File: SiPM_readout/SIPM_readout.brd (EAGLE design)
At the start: 57 x 37.5 mm, 28 parts

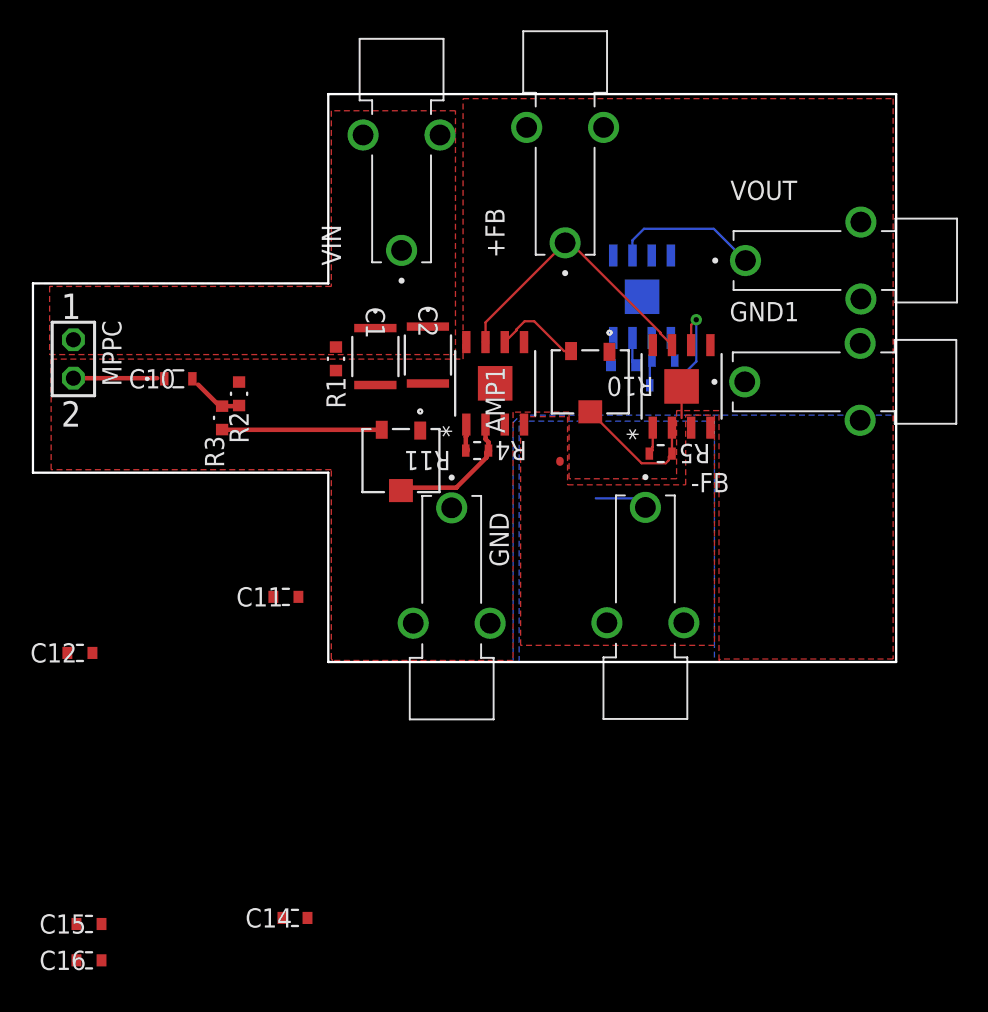
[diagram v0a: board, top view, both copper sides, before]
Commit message: compact
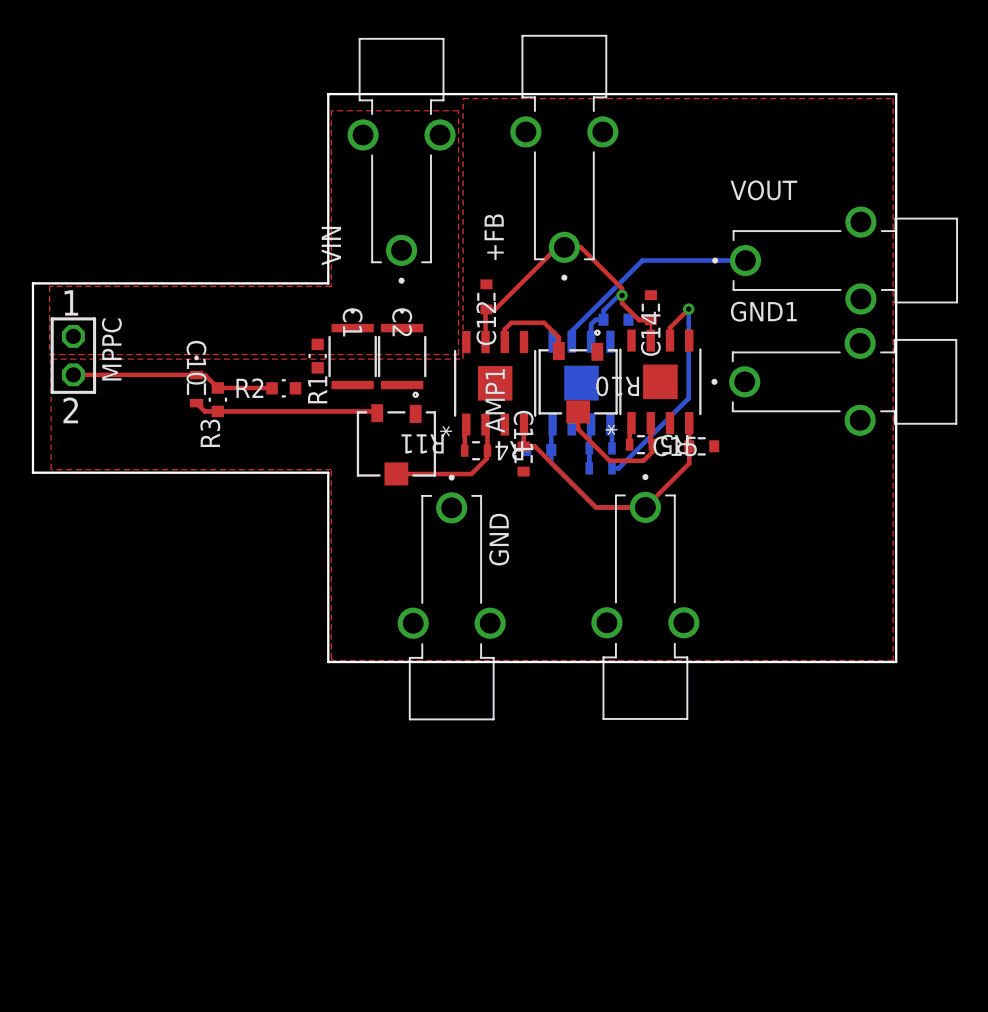
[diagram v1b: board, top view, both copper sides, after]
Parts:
- moved C16 54.8 mm to (47.5, 81.6), flipped to the bottom, turned to 180 degrees
- moved C15 51.3 mm to (53.2, 73.2)
- moved C14 46.7 mm to (49.8, 82.4), turned to 90 degrees
- moved C12 35.7 mm to (38.9, 83.1), turned to 90 degrees
- moved C11 18.1 mm to (41.4, 72.4), turned to 270 degrees
- moved C13 7.92 mm to (42.4, 73.0), turned to 0 degrees
- moved R6 7.12 mm to (46.5, 73.1)
- moved AMP3 6.96 mm to (45.2, 77.4)
- moved R9 6.78 mm to (46.5, 71.8)
- moved R2 2.97 mm to (25.6, 77.1), turned to 0 degrees
- moved C2 1.70 mm to (33.4, 79.2)
- moved C1 1.50 mm to (30.1, 79.2)
- moved AMP2 1.43 mm to (50.4, 77.5)
- moved R5 1.43 mm to (49.1, 73.3)
- moved C10 1.38 mm to (19.8, 77.0), turned to 270 degrees
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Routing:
- net -FB: track 5.84 -> 28.4 mm
- net N$18: track 6.79 -> 15.5 mm
- net N$2: track 8.93 -> 14.1 mm
- net VOUT: track 9.98 -> 14.4 mm
- net +FB: track 18.6 -> 23.0 mm, vias 0 -> 1
- net GND: track 4.50 -> 0.34 mm
- net N$3: track 10.6 -> 12.4 mm
- net N$16: track 0.00 -> 1.63 mm
- removed copper zone on layer 1, net -FB
- removed copper zone on layer 16, net -FB
